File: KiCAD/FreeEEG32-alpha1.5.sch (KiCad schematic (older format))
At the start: 109 parts, among them J59 Conn_01x03, J60 Conn_01x03, SW1 SW_Push, SW2 SW_Push

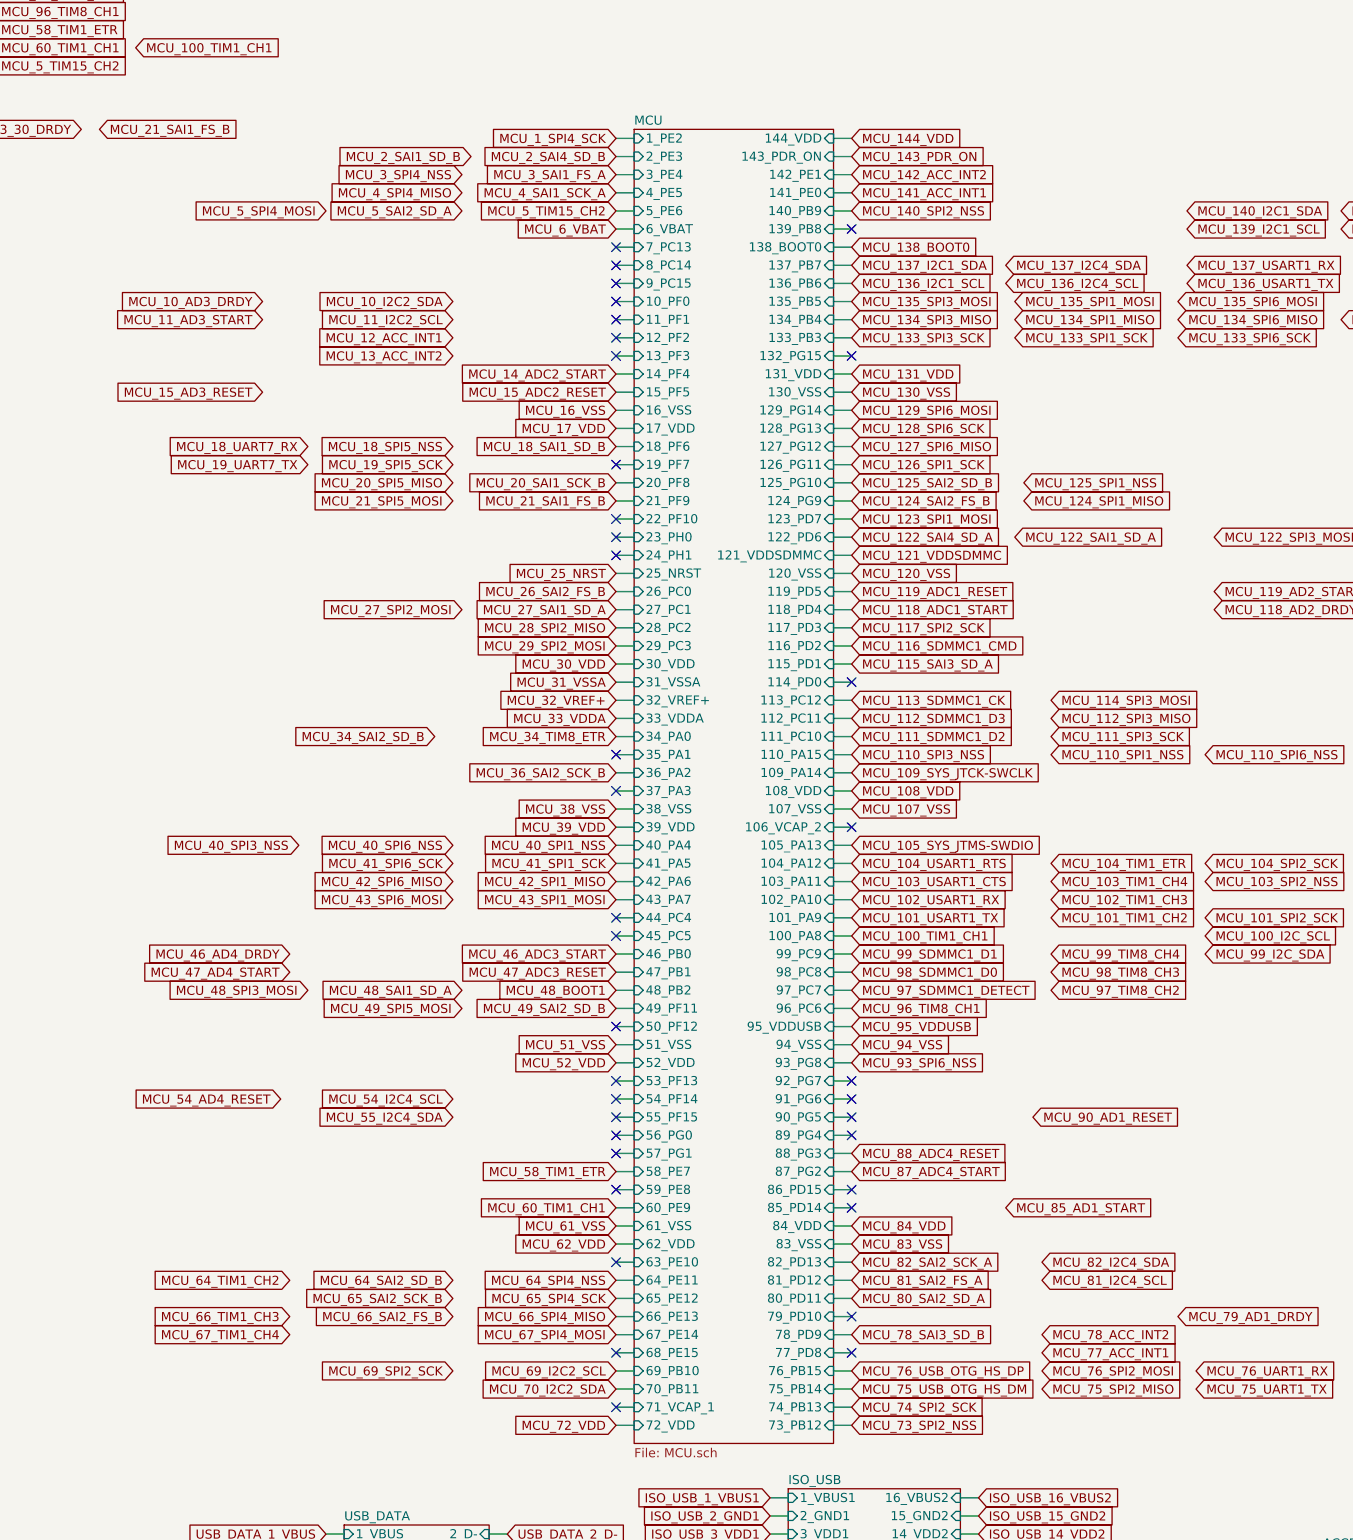
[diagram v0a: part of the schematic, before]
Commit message: Add files via upload
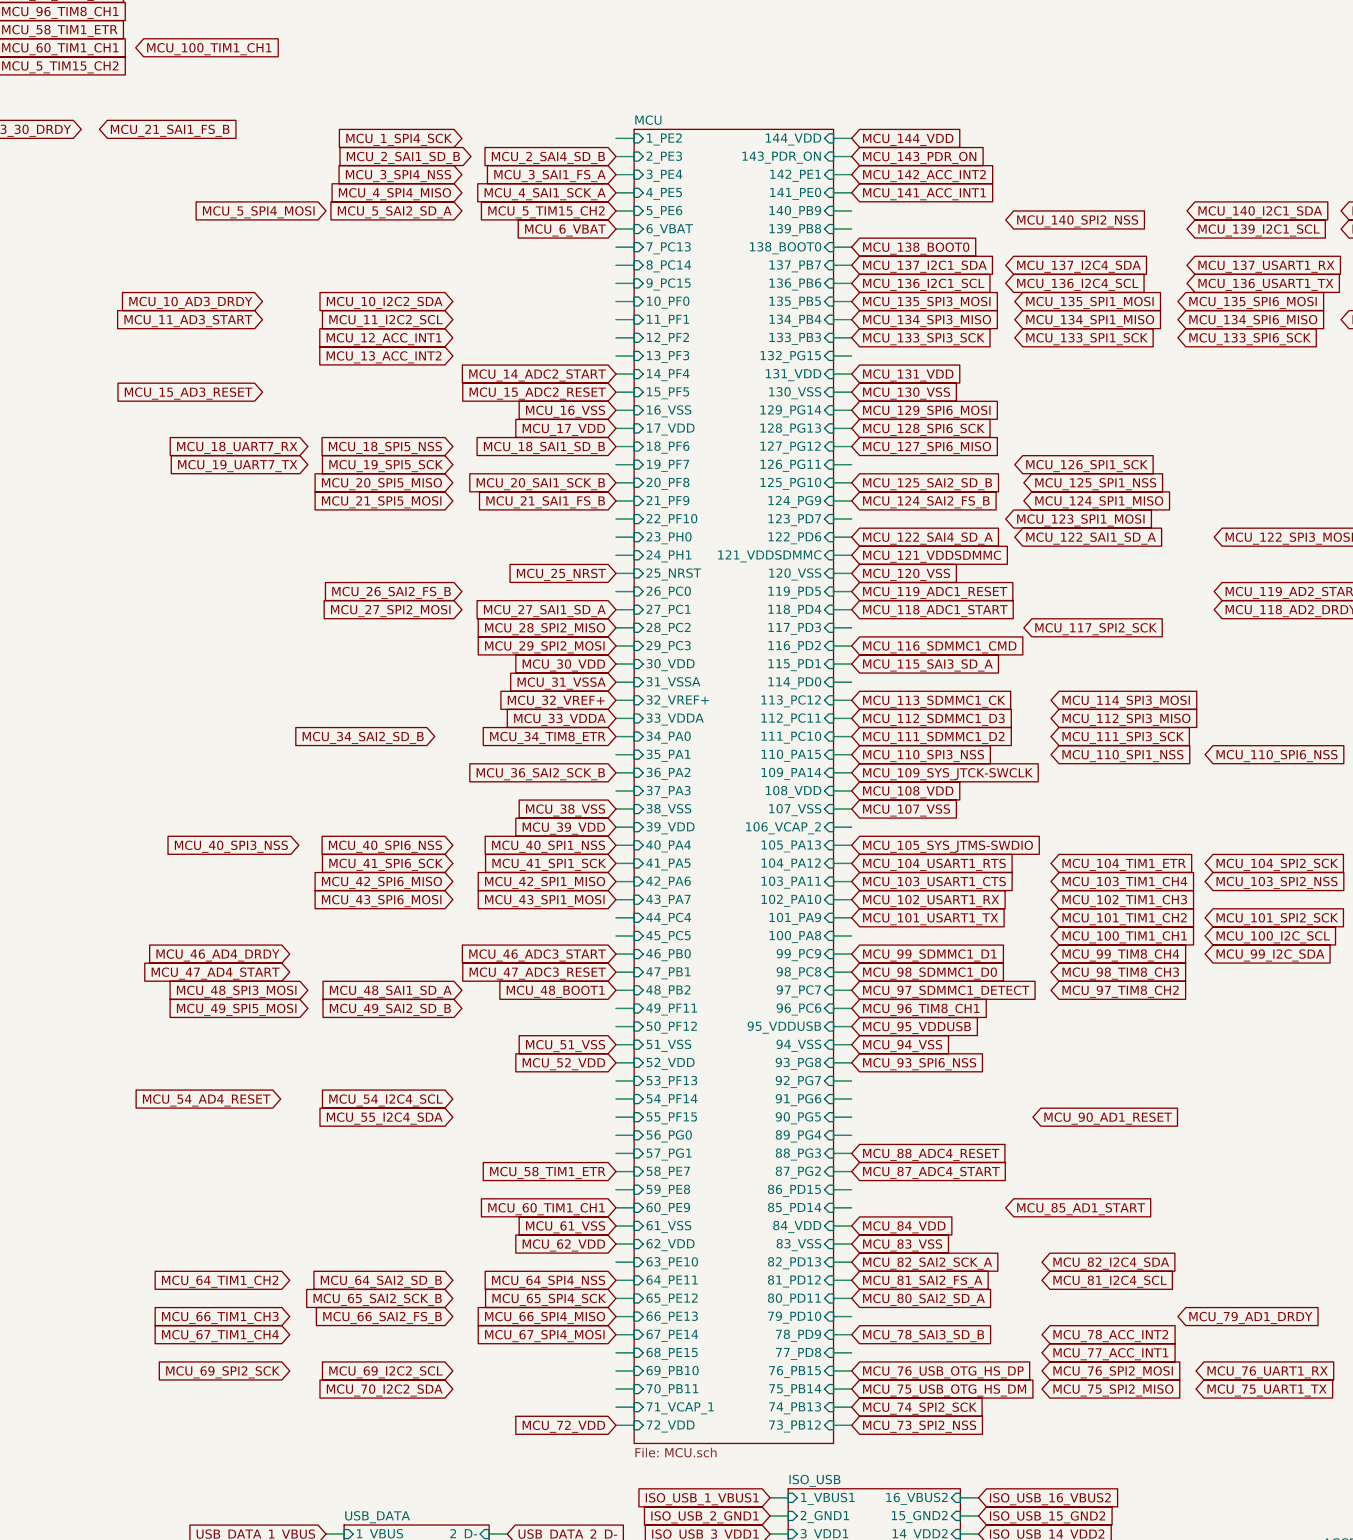
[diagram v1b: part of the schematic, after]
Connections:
- no-connect marks 159 -> 122
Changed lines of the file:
@@
 Wire Wire Line
 	1850 7650 1950 7650
-Text GLabel 650  7450 0    50   Input ~ 0
+Text GLabel -250 7450 0    50   Input ~ 0
 MCU_70_I2C2_SDA
 Wire Wire Line
 	650  7450 750  7450
-Text GLabel 650  7350 0    50   Input ~ 0
+Text GLabel -250 7350 0    50   Input ~ 0
 MCU_69_I2C2_SCL
 Text GLabel 650  7050 0    50   Input ~ 0
@@
 Wire Wire Line
 	650  3250 750  3250
-Text GLabel 650  3050 0    50   Input ~ 0
+Text GLabel -200 3050 0    50   Input ~ 0
 MCU_26_SAI2_FS_B
 Wire Wire Line
 	650  3050 750  3050
-Text GLabel 650  550  0    50   Input ~ 0
+Text GLabel -200 550  0    50   Input ~ 0
 MCU_1_SPI4_SCK
 Wire Wire Line
@@
 Text GLabel -1050 5250 0    50   Input ~ 0
 MCU_48_SPI3_MOSI
-Text GLabel 650  5350 0    50   Input ~ 0
-MCU_49_SAI2_SD_B
 Text GLabel -200 5350 0    50   Input ~ 0
+MCU_49_SAI2_SD_B
+Text GLabel -1050 5350 0    50   Input ~ 0
 MCU_49_SPI5_MOSI
 Text GLabel -250 5850 0    50   Input ~ 0
@@
 Text GLabel -1150 7150 0    50   Input ~ 0
 MCU_67_TIM1_CH4
-Text GLabel -250 7350 0    50   Input ~ 0
+Text GLabel -1150 7350 0    50   Input ~ 0
 MCU_69_SPI2_SCK
 Text GLabel 3000 7450 2    50   Input ~ 0
@@
 Text GLabel 3900 4950 2    50   Input ~ 0
 MCU_100_I2C_SCL
-Text GLabel 1950 4950 2    50   Input ~ 0
+Text GLabel 3050 4950 2    50   Input ~ 0
 MCU_100_TIM1_CH1
 Text GLabel 3050 4850 2    50   Input ~ 0
@@
 Text GLabel 3050 3650 2    50   Input ~ 0
 MCU_114_SPI3_MOSI
-Text GLabel 1950 3250 2    50   Input ~ 0
+Text GLabel 2900 3250 2    50   Input ~ 0
 MCU_117_SPI2_SCK
 Text GLabel 3950 2750 2    50   Input ~ 0
@@
 Text GLabel 2900 2450 2    50   Input ~ 0
 MCU_125_SPI1_NSS
-Text GLabel 1950 2650 2    50   Input ~ 0
+Text GLabel 2800 2650 2    50   Input ~ 0
 MCU_123_SPI1_MOSI
 Text GLabel 1950 2550 2    50   Input ~ 0
@@
 Text GLabel 2900 2550 2    50   Input ~ 0
 MCU_124_SPI1_MISO
-Text GLabel 1950 2350 2    50   Input ~ 0
+Text GLabel 2850 2350 2    50   Input ~ 0
 MCU_126_SPI1_SCK
 Text GLabel 2850 1650 2    50   Input ~ 0
@@
 Text GLabel 4650 950  2    50   Input ~ 0
 MCU_140_I2C4_SDA
-Text GLabel 1950 950  2    50   Input ~ 0
+Text GLabel 2800 1000 2    50   Input ~ 0
 MCU_140_SPI2_NSS
 Text GLabel -14450 -500 2    50   Input ~ 0
@@
 Wire Wire Line
 	650  7550 750  7550
-NoConn ~ 1950 7250
-NoConn ~ 1950 7050
-NoConn ~ 1950 6450
-NoConn ~ 1950 6350
-NoConn ~ 1950 6050
-NoConn ~ 1950 5950
-NoConn ~ 1950 5850
-NoConn ~ 1950 5750
-NoConn ~ 650  5750
-NoConn ~ 650  5850
-NoConn ~ 650  5950
-NoConn ~ 650  6050
-NoConn ~ 650  6150
-NoConn ~ 650  6350
-NoConn ~ 650  6750
-NoConn ~ 650  7250
-NoConn ~ 650  7550
-NoConn ~ 650  5450
-NoConn ~ 1950 4350
-NoConn ~ 1950 3550
-NoConn ~ 650  3950
-NoConn ~ 650  4150
-NoConn ~ 650  4850
-NoConn ~ 650  4950
-NoConn ~ 650  2650
-NoConn ~ 650  2750
-NoConn ~ 650  2850
-NoConn ~ 650  2350
-NoConn ~ 650  1150
-NoConn ~ 650  1250
-NoConn ~ 650  1350
-NoConn ~ 650  1450
-NoConn ~ 650  1550
-NoConn ~ 1950 1050
-NoConn ~ 650  1750
-NoConn ~ 650  1650
-NoConn ~ 1950 1750
 Text GLabel 8400 1950 0    50   Input ~ 0
 ADC4_13_MODE0_GPIO0

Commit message: Add files via upload
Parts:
- added J65, J69, J73, J77, J78, J79, J80, J81, J84, J85, J86, J87: Conn_01x02, Connector_PinSocket_2.54mm:PinSocket_1x02_P2.54mm_Vertical, symbol Connector_Generic:Conn_01x02
- added J66, J67, J68: Conn_01x02, Connector_PinSocket_1.27mm:PinSocket_1x02_P1.27mm_Vertical, symbol Connector_Generic:Conn_01x02
- added J70, J71, J72, J74, J75, J76: Conn_01x02, symbol Connector_Generic:Conn_01x02
- added J82, J83: Conn_02x02_Odd_Even, Connector_PinSocket_2.54mm:PinSocket_2x02_P2.54mm_Horizontal, symbol Connector_Generic:Conn_02x02_Odd_Even
- added R110, R111, R112, R113, R114, R115, R116, R117: 0, Resistor_SMD:R_0402_1005Metric, symbol Device:R_Small
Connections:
- net labels added: ADC2_13_MODE0_GPIO1, ADC2_35_SYNC_OUT, ADC3_13_MODE0_GPIO1, ADC3_35_SYNC_OUT, ADC4_13_MODE0_GPIO1, ADC4_35_SYNC_OUT, MCU_100_PA8_TIM1_CH1, MCU_101_PA9_USART1_TX, MCU_102_PA10_USART1_RX, MCU_103_PA11_USART1_CTS, MCU_104_PA12_USART1_RTS, MCU_105_PA13_SYS_JTMS-SWDIO, MCU_109_PA14_SYS_JTCK-SWCLK, MCU_10_PF0_I2C2_SDA, MCU_110_PA15_SPI3_NSS, MCU_111_PC10_SDMMC1_D2, MCU_112_PC11_SDMMC1_D3, MCU_113_PC12_SDMMC1_CK, MCU_114_SDMMC1_DETECT, MCU_115_PD1_SAI3_SD_A, MCU_116_PD2_SDMMC1_CMD, MCU_117_PD3_SPI2_SCK, MCU_118_PD4_ADC1_START, MCU_119_PD5_ADC1_RESET, MCU_11_PF1_I2C2_SCL, MCU_122_PD6_SAI4_SD_A, MCU_124_PG9_SAI2_FS_B, MCU_125_PG10_SAI2_SD_B, MCU_127_PG12_SPI6_MISO, MCU_128_PG13_SPI6_SCK, MCU_129_PG14_SPI6_MOSI, MCU_133_PB3_SPI3_SCK, MCU_134_PB4_SPI3_MISO, MCU_135_PB5_SPI3_MOSI, MCU_136_PB6_I2C1_SCL, MCU_137_PB7_I2C1_SDA, MCU_141_PE0_ACC_INT1, MCU_142_PE1_ACC_INT2, MCU_14_PF4_ADC2_START, MCU_15_PF5_ADC2_RESET, MCU_18_PF6_SAI1_SD_B, MCU_20_PF8_SAI1_SCK_B, MCU_21_PF9_SAI1_FS_B, MCU_22_PF10, MCU_22_PF10_ADC3_DRDY, MCU_27_PC1_SAI1_SD_A, MCU_28_PC2_SPI2_MISO, MCU_29_PC3_SPI2_MOSI, MCU_2_PE3_SAI4_SD_B, MCU_34_PA0_TIM8_ETR, MCU_36_PA2_SAI2_SCK_B, MCU_3_PE4, MCU_3_PE4_SAI1_FS_A, MCU_40_PA4_SPI1_NSS, MCU_41_PA5_SPI1_SCK, MCU_42_PA6_SPI1_MISO, MCU_43_PA7_SPI1_MOSI, MCU_46_PB0_ADC3_START, MCU_47_PB1_ADC3_RESET, MCU_48_PB2_BOOT1, MCU_4_PE5_SAI1_SCK_A, MCU_54_PF14_I2C4_SCL, MCU_55_PF15_I2C4_SDA, MCU_58_PE7_TIM1_ETR, MCU_5_PE6_TIM15_CH2, MCU_60_PE9_TIM1_CH1, MCU_64_PE11_SPI4_NSS, MCU_64_PE11_TIM1_CH2, MCU_65_PE12_SPI4_SCK, MCU_66_PE13_SPI4_MISO, MCU_67_PE14_SPI4_MOSI, MCU_69_PB10_I2C2_SCL, MCU_69_PB10_USART3_RX, MCU_70_PB11_I2C2_SDA, MCU_70_PB11_USART3_TX, MCU_73_PB12_SPI2_NSS, MCU_74_PB13_SPI2_SCK, MCU_75_PB14_USB_OTG_HS_DM, MCU_76_PB15_USB_OTG_HS_DP, MCU_78_PD9_SAI3_SD_B, MCU_7_PC13, MCU_7_PC13_ADC2_DRDY, MCU_80_PD11_SAI2_SD_A, MCU_81_P12_SAI2_FS_A, MCU_82_PD13_SAI2_SCK_A, MCU_87_PG2_ADC4_START, MCU_88_PG3_ADC4_RESET, MCU_89_PG4_ADC4_DRDY, MCU_90_PG5, MCU_90_PG5_ADC1_DRDY, MCU_93_PG8_SPI6_NSS, MCU_96_PC6_TIM8_CH1, MCU_97_PC7_SDMMC1_DETECT, MCU_97_PC7_TIM8_CH2, MCU_98_PC8_SDMMC1_D0, MCU_99_PC9_SDMMC1_D1
- net labels removed: MCU_101_USART1_TX, MCU_102_USART1_RX, MCU_103_USART1_CTS, MCU_104_USART1_RTS, MCU_111_SDMMC1_D2, MCU_112_SDMMC1_D3, MCU_113_SDMMC1_CK, MCU_115_SAI3_SD_A, MCU_116_SDMMC1_CMD, MCU_118_ADC1_START, MCU_119_ADC1_RESET, MCU_122_SAI4_SD_A, MCU_136_I2C1_SCL, MCU_137_I2C1_SDA, MCU_141_ACC_INT1, MCU_142_ACC_INT2, MCU_14_ADC2_START, MCU_15_ADC2_RESET, MCU_2_SAI4_SD_B, MCU_34_TIM8_ETR, MCU_46_ADC3_START, MCU_47_ADC3_RESET, MCU_48_BOOT1, MCU_54_I2C4_SCL, MCU_55_I2C4_SDA, MCU_58_TIM1_ETR, MCU_60_TIM1_CH1, MCU_75_USB_OTG_HS_DM, MCU_76_USB_OTG_HS_DP, MCU_78_SAI3_SD_B, MCU_87_ADC4_START, MCU_88_ADC4_RESET, MCU_96_TIM8_CH1, MCU_97_SDMMC1_DETECT, MCU_98_SDMMC1_D0, MCU_99_SDMMC1_D1
- wire segments 847 -> 937
- no-connect marks 122 -> 150
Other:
- moved on the sheet: R103, R104, R105, R106, R107, R65, R66, R67, R68, R69, R70, R71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

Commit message: Add files via upload
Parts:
- added J88: Conn_01x02, Connector_PinSocket_2.54mm:PinSocket_1x02_P2.54mm_Vertical, symbol Connector_Generic:Conn_01x02
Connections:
- net labels added: ADC1_57_VCM, ADC2_57_VCM, ADC3_57_VCM, ADC4_57_VCM, AINREF-, MCU_114_PD0_ADC1_DRDY, MCU_139_PB8_ACC_INT1, MCU_140_PB9_ACC_SDO_SAO, MCU_19_PF7_ISO_USB_PIN, MCU_45_PC5_ADC3_START, MCU_46_PB0_ADC1_DRDY, VCM
- wire segments 937 -> 953
- no-connect marks 150 -> 147

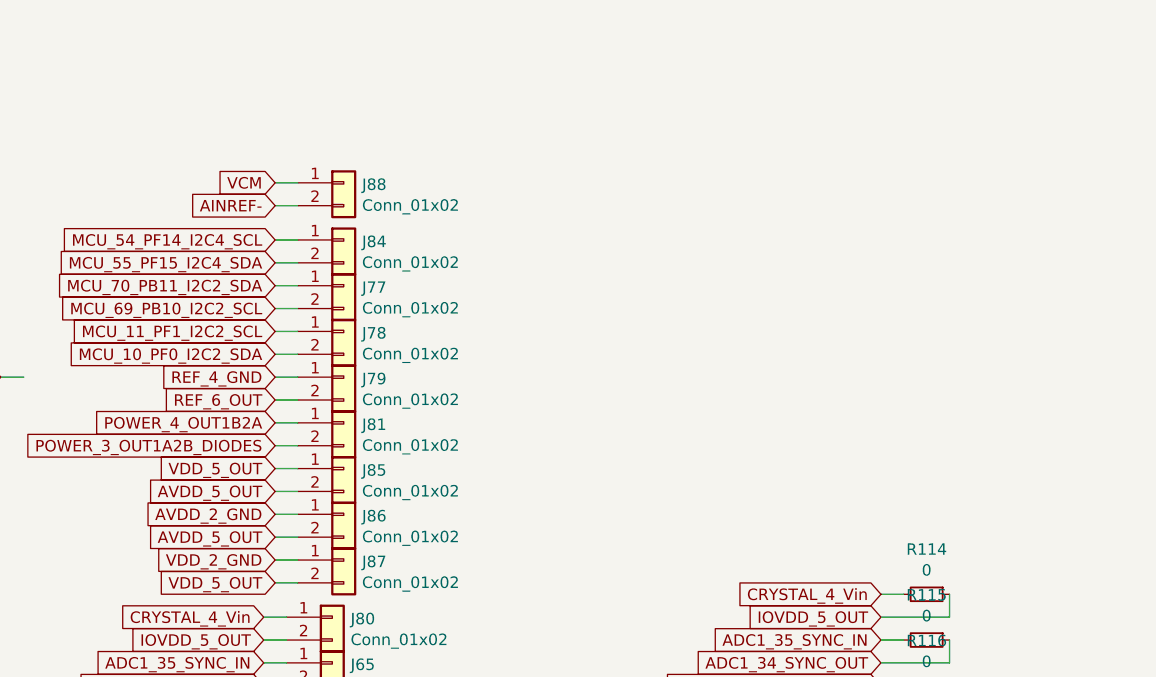
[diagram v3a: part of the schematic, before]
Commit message: Add files via upload
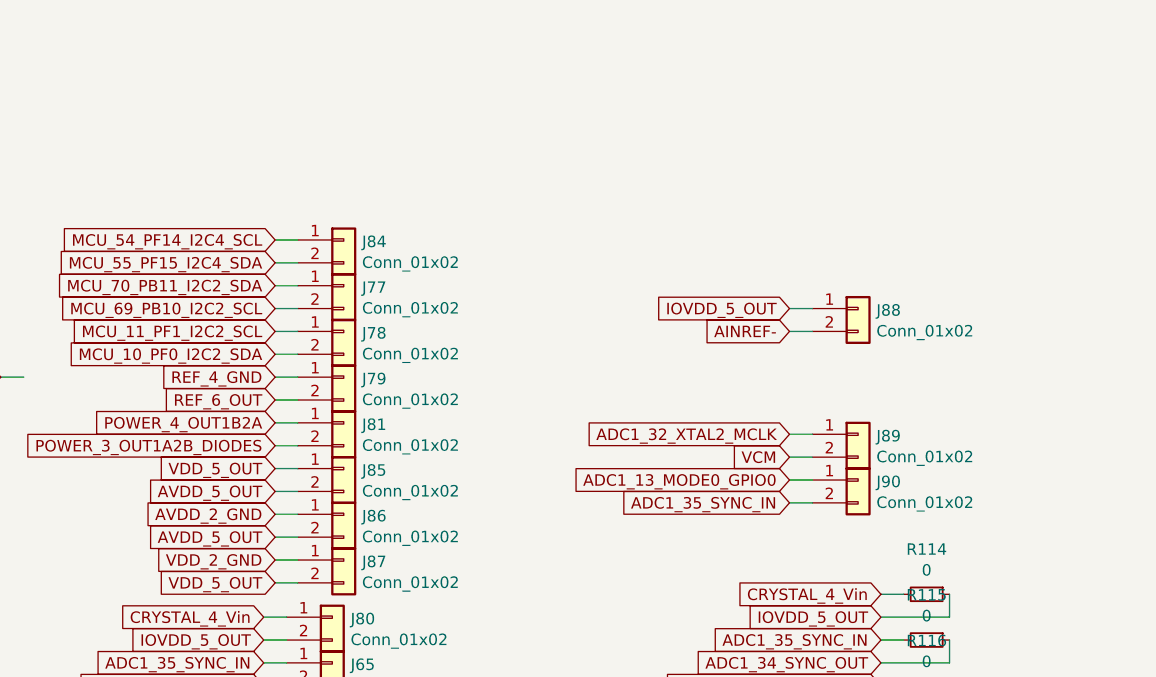
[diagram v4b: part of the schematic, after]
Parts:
- added J89, J90: Conn_01x02, Connector_PinSocket_2.54mm:PinSocket_1x02_P2.54mm_Vertical, symbol Connector_Generic:Conn_01x02
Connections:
- wire segments 953 -> 957
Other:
- moved on the sheet: J88
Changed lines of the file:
@@
 L Connector_Generic:Conn_01x02 J88
 U 1 1 5D6671F5
-P 14350 -4400
-F 0 "J88" H 14430 -4408 50  0000 L CNN
-F 1 "Conn_01x02" H 14430 -4499 50  0000 L CNN
-F 2 "Connector_PinSocket_2.54mm:PinSocket_1x02_P2.54mm_Vertical" H 14350 -4400 50  0001 C CNN
-F 3 "~" H 14350 -4400 50  0001 C CNN
-	1    14350 -4400
+P 16600 -3850
+F 0 "J88" H 16680 -3858 50  0000 L CNN
+F 1 "Conn_01x02" H 16680 -3949 50  0000 L CNN
+F 2 "Connector_PinSocket_2.54mm:PinSocket_1x02_P2.54mm_Vertical" H 16600 -3850 50  0001 C CNN
+F 3 "~" H 16600 -3850 50  0001 C CNN
+	1    16600 -3850
 	1    0    0    -1
 $EndComp
 Wire Wire Line
-	14150 -4300 14050 -4300
+	16400 -3750 16300 -3750
 Wire Wire Line
-	14150 -4400 14050 -4400
-Text GLabel 14050 -4400 0    50   Input ~ 0
+	16400 -3200 16300 -3200
+Text GLabel 16300 -3200 0    50   Input ~ 0
 VCM
-Text GLabel 14050 -4300 0    50   Input ~ 0
+Text GLabel 16300 -3750 0    50   Input ~ 0
 AINREF-
 Text GLabel 16550 900  2    50   Input ~ 0
@@
 Text GLabel -3300 6300 2    50   Input ~ 0
 MCU_19_PF7_ISO_USB_PIN
+$Comp
+L Connector_Generic:Conn_01x02 J89
+U 1 1 5D6C1D06
+P 16600 -3300
+F 0 "J89" H 16680 -3308 50  0000 L CNN
+F 1 "Conn_01x02" H 16680 -3399 50  0000 L CNN
+F 2 "Connector_PinSocket_2.54mm:PinSocket_1x02_P2.54mm_Vertical" H 16600 -3300 50  0001 C CNN
+F 3 "~" H 16600 -3300 50  0001 C CNN
+	1    16600 -3300
+	1    0    0    -1
+$EndComp
+Text GLabel 16300 -3300 0    50   Input ~ 0
+ADC1_32_XTAL2_MCLK
+Text GLabel 16300 -3100 0    50   Input ~ 0
+ADC1_13_MODE0_GPIO0
+$Comp
+L Connector_Generic:Conn_01x02 J90
+U 1 1 5D6C2072
+P 16600 -3100
+F 0 "J90" H 16680 -3108 50  0000 L CNN
+F 1 "Conn_01x02" H 16680 -3199 50  0000 L CNN
+F 2 "Connector_PinSocket_2.54mm:PinSocket_1x02_P2.54mm_Vertical" H 16600 -3100 50  0001 C CNN
+F 3 "~" H 16600 -3100 50  0001 C CNN
+	1    16600 -3100
+	1    0    0    -1
+$EndComp
+Text GLabel 16300 -3000 0    50   Input ~ 0
+ADC1_35_SYNC_IN
+Text GLabel 16300 -3850 0    50   Input ~ 0
+IOVDD_5_OUT
+Wire Wire Line
+	16300 -3300 16400 -3300
+Wire Wire Line
+	16300 -3850 16400 -3850
+Wire Wire Line
+	16300 -3100 16400 -3100
+Wire Wire Line
+	16300 -3000 16400 -3000
 $EndSCHEMATC
